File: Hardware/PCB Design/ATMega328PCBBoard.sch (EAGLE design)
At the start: 14 parts

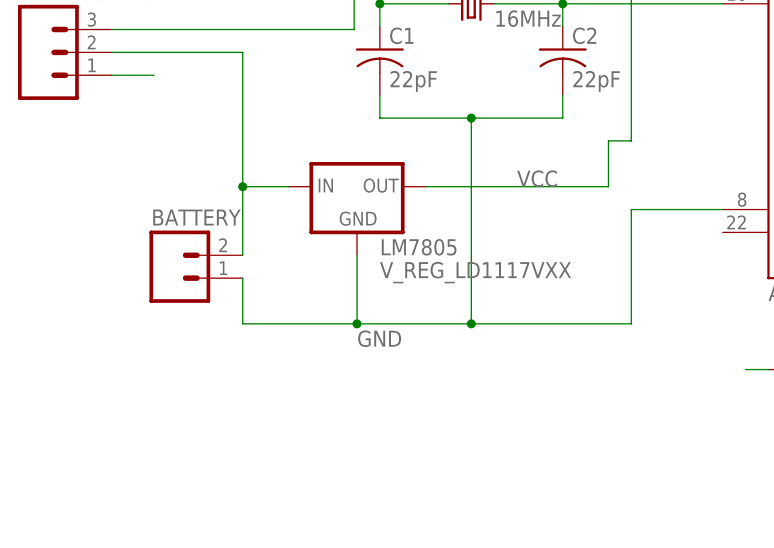
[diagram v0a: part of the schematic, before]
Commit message: final board design
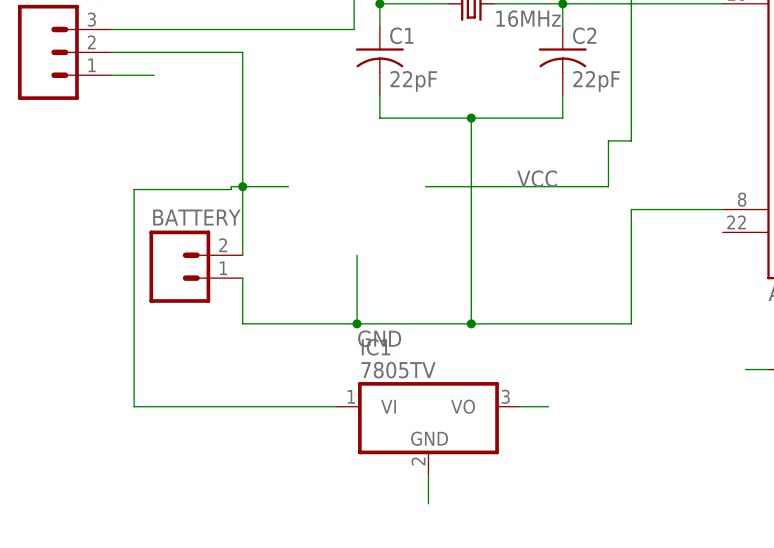
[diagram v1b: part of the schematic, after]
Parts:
- removed LM7805: V_REG_LD1117VXX, SparkFun-PowerIC:V_REG_LD1117VXX
- added IC1: 7805TV, linear:7805TV
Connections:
- net GND: now also IC1.GND; no longer LM7805.GND
- net N$4: now also IC1.VI; no longer LM7805.IN
- net VCC: now also IC1.VO; no longer LM7805.OUT
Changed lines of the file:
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@@
 <part name="C1" library="adafruit" deviceset="C-US" device="050-025X075" value="22pF"/>
 <part name="C2" library="adafruit" deviceset="C-US" device="050-025X075" value="22pF"/>
-<part name="LM7805" library="SparkFun-PowerIC" deviceset="V_REG_LD1117VXX" device=""/>
 <part name="MOTOR" library="SparkFun-Connectors" deviceset="M04" device="JST"/>
 <part name="R1" library="resistor" deviceset="R-US_" device="0207/2V" value="220"/>
@@
 <part name="LOAD" library="SparkFun-Connectors" deviceset="M02" device="JST-PTH-VERT"/>
 <part name="3.3REGULATOR" library="SparkFun-Connectors" deviceset="M03" device="JST-PTH-VERT"/>
+<part name="IC1" library="linear" deviceset="78*" device="TV" technology="05"/>
 </parts>
 <sheets>
@@
 <instance part="C1" gate="G$1" x="-12.7" y="48.26"/>
 <instance part="C2" gate="G$1" x="7.62" y="48.26"/>
-<instance part="LM7805" gate="G$1" x="-15.24" y="33.02"/>
 <instance part="MOTOR" gate="G$1" x="106.68" y="66.04" rot="R180"/>
 <instance part="R1" gate="G$1" x="35.56" y="12.7"/>
@@
 <instance part="LOAD" gate="G$1" x="5.08" y="86.36"/>
 <instance part="3.3REGULATOR" gate="G$1" x="-50.165" y="47.9425"/>
+<instance part="IC1" gate="A1" x="-7.3025" y="8.5725"/>
 </instances>
 <busses>
@@
 <net name="VCC" class="0">
 <segment>
-<pinref part="LM7805" gate="G$1" pin="OUT"/>
 <wire x1="-7.62" y1="33.02" x2="12.7" y2="33.02" width="0.1524" layer="91"/>
 <wire x1="12.7" y1="33.02" x2="12.7" y2="38.1" width="0.1524" layer="91"/>
@@
 <wire x1="101.6" y1="68.58" x2="99.06" y2="68.58" width="0.1524" layer="91"/>
 </segment>
+<segment>
+<pinref part="IC1" gate="A1" pin="VO"/>
+<wire x1="2.8575" y1="8.5725" x2="6.0325" y2="8.5725" width="0.1524" layer="91"/>
+</segment>
 </net>
 <net name="A0" class="0">
@@
 <junction x="-2.54" y="40.64"/>
 <wire x1="-27.94" y1="17.78" x2="-15.24" y2="17.78" width="0.1524" layer="91"/>
-<pinref part="LM7805" gate="G$1" pin="GND"/>
 <wire x1="-15.24" y1="17.78" x2="-15.24" y2="25.4" width="0.1524" layer="91"/>
 <wire x1="-15.24" y1="17.78" x2="-2.54" y2="17.78" width="0.1524" layer="91"/>
@@
 <wire x1="-42.545" y1="45.4025" x2="-37.7825" y2="45.4025" width="0.1524" layer="91"/>
 </segment>
+<segment>
+<pinref part="IC1" gate="A1" pin="GND"/>
+<wire x1="-7.3025" y1="0.9525" x2="-7.3025" y2="-2.2225" width="0.1524" layer="91"/>
+</segment>
 </net>
 <net name="3VCC" class="0">
@@
 <segment>
 <pinref part="3.3REGULATOR" gate="G$1" pin="2"/>
-<pinref part="LM7805" gate="G$1" pin="IN"/>
 <wire x1="-27.94" y1="33.02" x2="-22.86" y2="33.02" width="0.1524" layer="91"/>
 <pinref part="BATTERY" gate="G$1" pin="2"/>
@@
 <wire x1="-42.545" y1="47.9425" x2="-27.94" y2="47.9425" width="0.1524" layer="91"/>
 <wire x1="-27.94" y1="47.9425" x2="-27.94" y2="33.02" width="0.1524" layer="91"/>
-</segment>
-</net>
+<pinref part="IC1" gate="A1" pin="VI"/>
+<wire x1="-17.4625" y1="8.5725" x2="-40.005" y2="8.5725" width="0.1524" layer="91"/>
+<wire x1="-40.005" y1="8.5725" x2="-40.005" y2="32.7025" width="0.1524" layer="91"/>
+<wire x1="-40.005" y1="32.7025" x2="-29.21" y2="32.7025" width="0.1524" layer="91"/>
+<wire x1="-29.21" y1="32.7025" x2="-29.21" y2="33.02" width="0.1524" layer="91"/>
+<wire x1="-29.21" y1="33.02" x2="-27.94" y2="33.02" width="0.1524" layer="91"/>
+</segment>
+</net>
